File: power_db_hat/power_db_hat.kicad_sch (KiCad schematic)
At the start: 27 parts, among them J2 BAT1, J3 12V_out, J4 Conn_01x04_Pin, J5 24V_out, J6 PD_power, J7 Conn_01x20_Pin, J8 BAT2

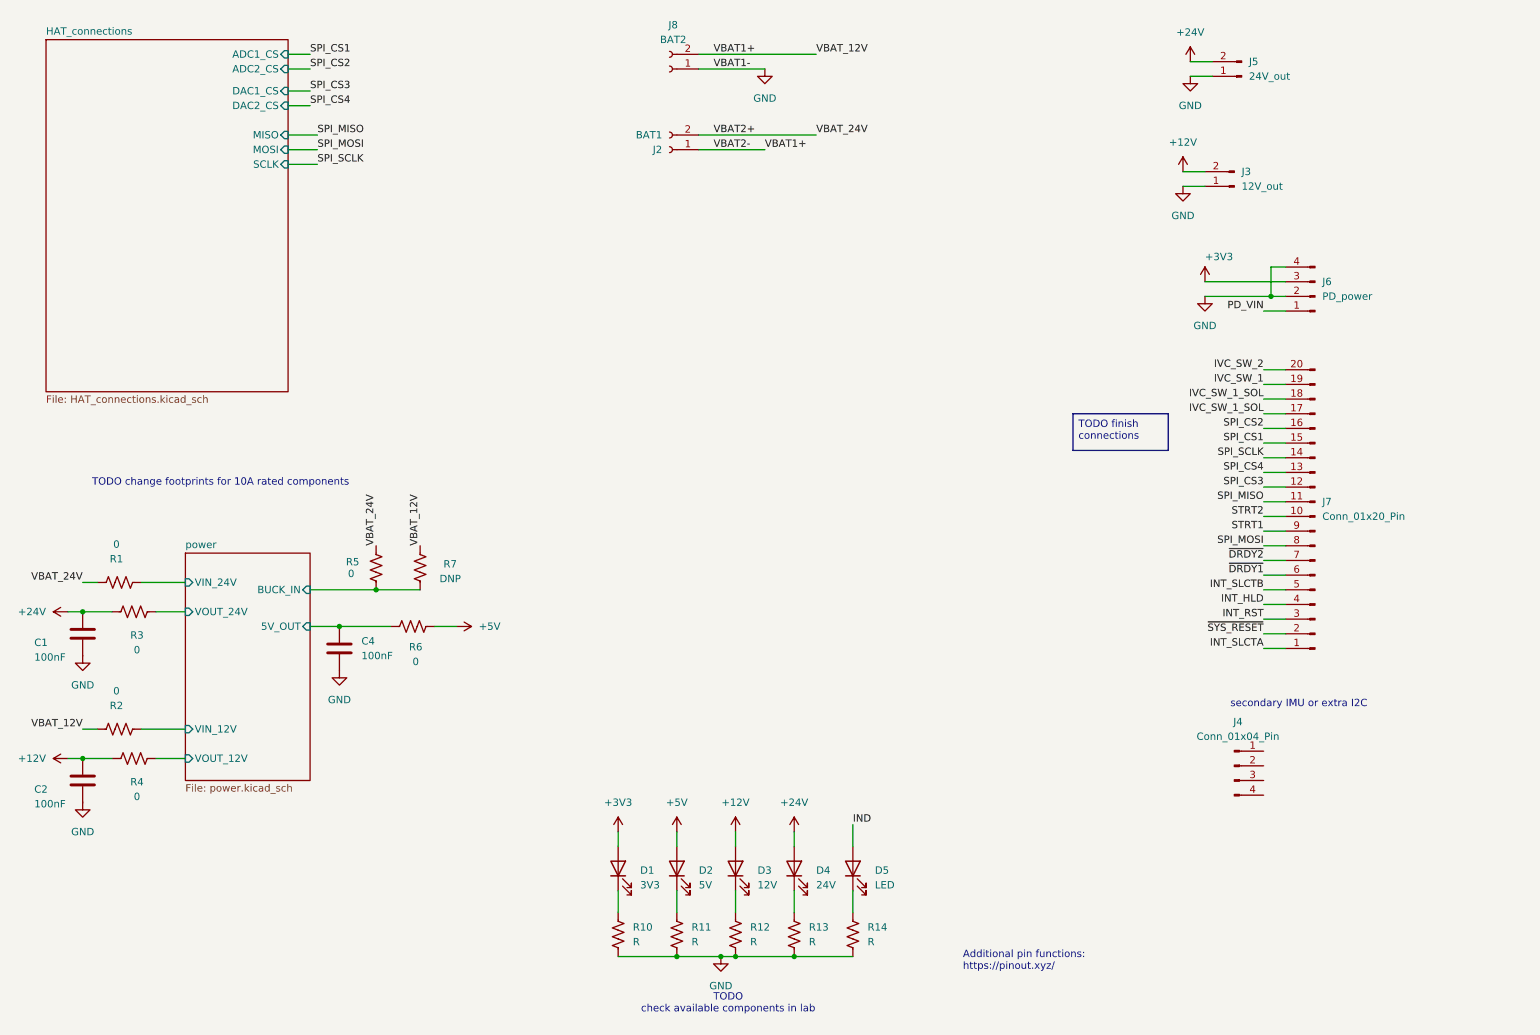
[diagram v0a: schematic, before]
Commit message: update
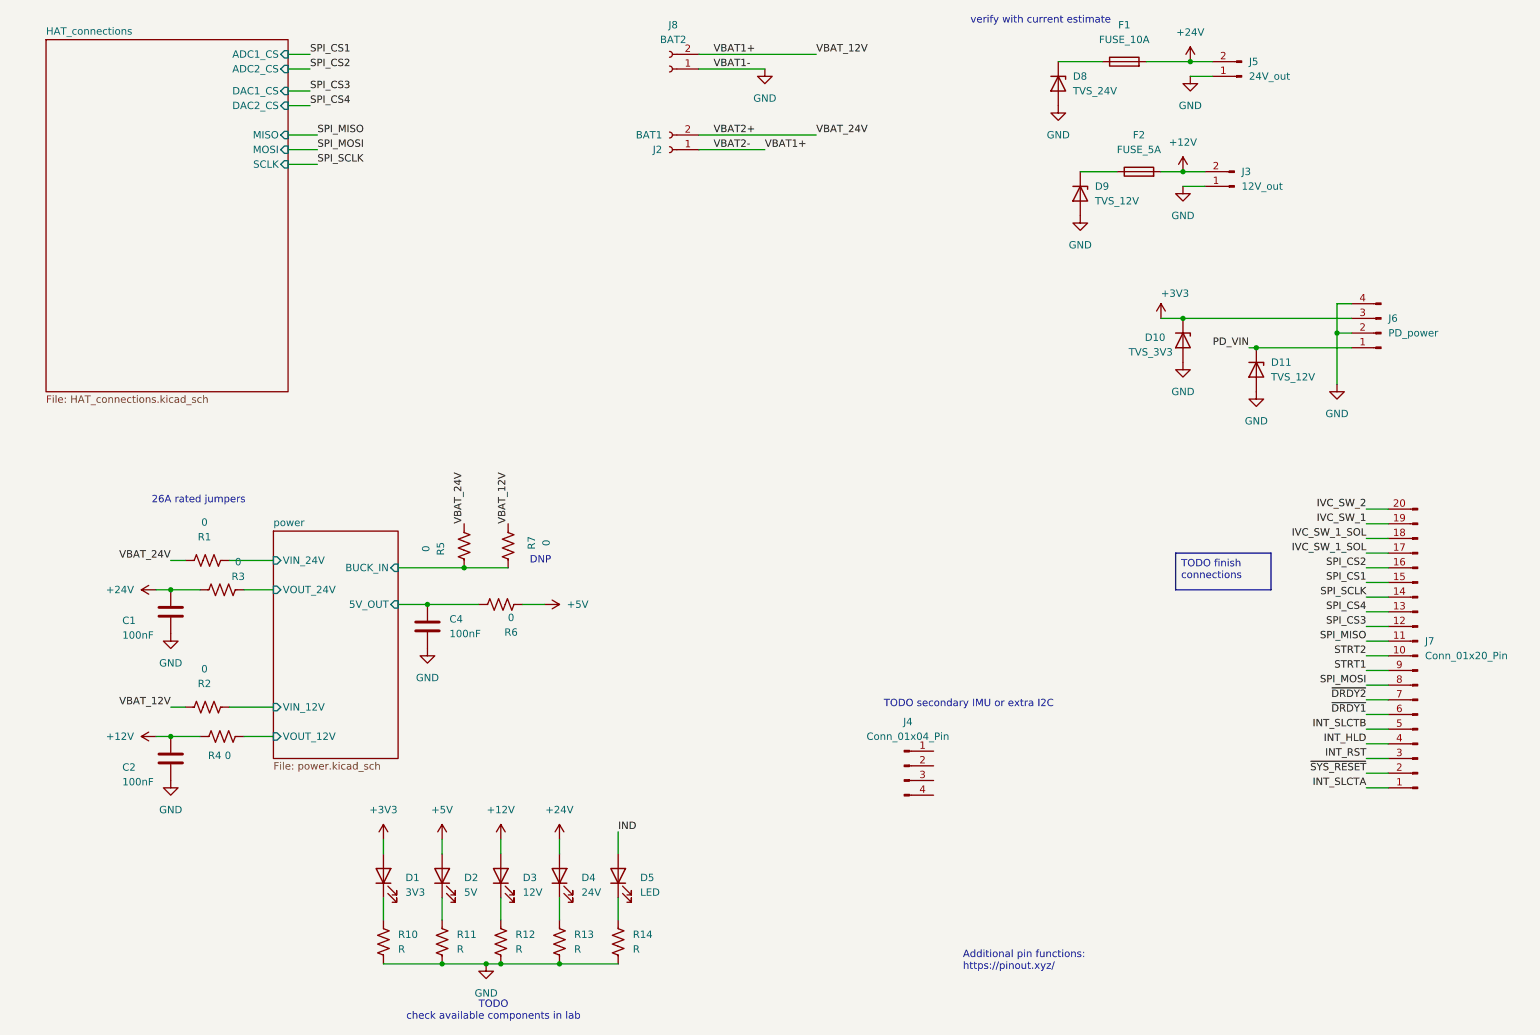
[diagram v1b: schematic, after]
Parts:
- added D10: TVS_3V3, symbol Device:D_Zener
- added D11, D9: TVS_12V, symbol Device:D_Zener
- added D8: TVS_24V, symbol Device:D_Zener
- added F1: FUSE_10A, symbol Device:Fuse
- added F2: FUSE_5A, symbol Device:Fuse
- R7: value DNP -> 0
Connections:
- net +12V: now also R4.2, F2.2; no longer R4.1
- net +24V: now also R3.2, F1.2; no longer R3.1
- net +3V3: now also D10.1 (K)
- net +5V: now also R6.1; no longer R6.2
- net GND: now also D10.2 (A), D11.2 (A), D8.2 (A), D9.2 (A)
- net PD_VIN: now also D11.1 (K)
- net VBAT1+: now also R7.2; no longer R7.1
- net power/5V_OUT: now also R6.2; no longer R6.1
- net power/BUCK_IN: now also R7.1; no longer R7.2
- net power/VOUT_12V: now also R4.1; no longer R4.2
- net power/VOUT_24V: now also R3.1; no longer R3.2
- new net: D8.1 (K), F1.1
- new net: D9.1 (K), F2.1
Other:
- note added: "26A rated jumpers"
- note added: "DNP"
- note added: "TODO secondary IMU or extra I2C"
- note added: "verify with current estimate"
- note removed: "TODO change footprints for 10A rated components"
- note removed: "secondary IMU or extra I2C"
- moved on the sheet: C1, C2, C4, D1, D2, D3, D4, D5, J4, J6, J7, R1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
